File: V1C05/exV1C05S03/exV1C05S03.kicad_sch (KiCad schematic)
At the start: 4 parts

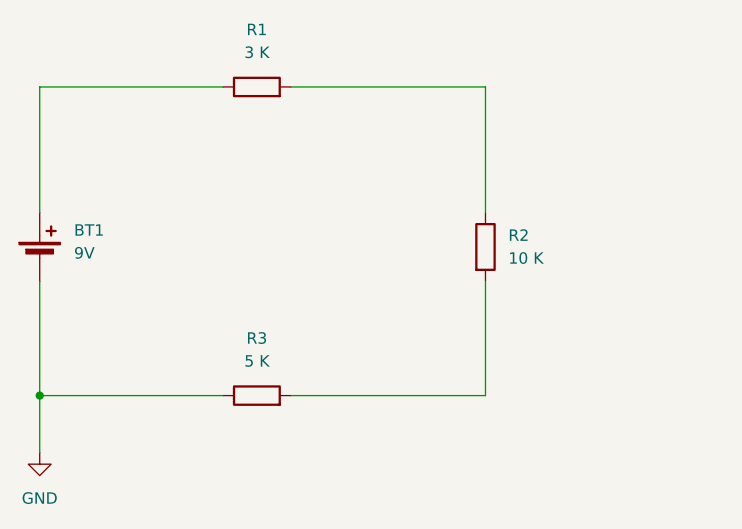
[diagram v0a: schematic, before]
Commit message: update exV1C05S03
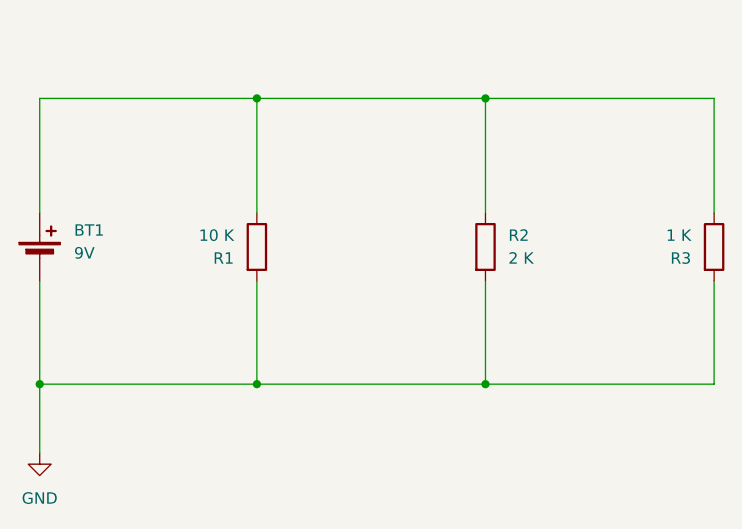
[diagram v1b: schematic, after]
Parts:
- R1: value 3 K -> 10 K
- R2: value 10 K -> 2 K
- R3: value 5 K -> 1 K
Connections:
- net GND: now also R1.2, R2.2, R3.2; no longer R3.1
- net at R2.1: now also BT1.1 (+), R1.1, R3.1; no longer R1.2
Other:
- moved on the sheet: R1, R3
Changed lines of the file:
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@@
 	(paper "A4")
 	(junction
-		(at 44.45 60.96)
-		(diameter 0)
-		(color 0 0 0 0)
-	)
-	(wire
-		(pts
-			(xy 72.39 26.67) (xy 93.98 26.67)
-		)
-		(stroke
-			(width 0)
-			(type default)
-		)
-	)
-	(wire
-		(pts
-			(xy 72.39 60.96) (xy 93.98 60.96)
-		)
-		(stroke
-			(width 0)
-			(type default)
-		)
-	)
-	(wire
-		(pts
-			(xy 44.45 60.96) (xy 64.77 60.96)
-		)
-		(stroke
-			(width 0)
-			(type default)
-		)
-	)
-	(wire
-		(pts
-			(xy 93.98 48.26) (xy 93.98 60.96)
-		)
-		(stroke
-			(width 0)
-			(type default)
-		)
-	)
-	(wire
-		(pts
-			(xy 44.45 48.26) (xy 44.45 60.96)
-		)
-		(stroke
-			(width 0)
-			(type default)
-		)
-	)
-	(wire
-		(pts
-			(xy 93.98 26.67) (xy 93.98 40.64)
-		)
-		(stroke
-			(width 0)
-			(type default)
-		)
-	)
-	(wire
-		(pts
-			(xy 44.45 60.96) (xy 44.45 67.31)
-		)
-		(stroke
-			(width 0)
-			(type default)
-		)
-	)
-	(wire
-		(pts
-			(xy 44.45 26.67) (xy 64.77 26.67)
-		)
-		(stroke
-			(width 0)
-			(type default)
-		)
-	)
-	(wire
-		(pts
-			(xy 44.45 40.64) (xy 44.45 26.67)
+		(at 68.58 27.94)
+		(diameter 0)
+		(color 0 0 0 0)
+	)
+	(junction
+		(at 68.58 59.69)
+		(diameter 0)
+		(color 0 0 0 0)
+	)
+	(junction
+		(at 44.45 59.69)
+		(diameter 0)
+		(color 0 0 0 0)
+	)
+	(junction
+		(at 93.98 59.69)
+		(diameter 0)
+		(color 0 0 0 0)
+	)
+	(junction
+		(at 93.98 27.94)
+		(diameter 0)
+		(color 0 0 0 0)
+	)
+	(wire
+		(pts
+			(xy 119.38 59.69) (xy 93.98 59.69)
+		)
+		(stroke
+			(width 0)
+			(type default)
+		)
+	)
+	(wire
+		(pts
+			(xy 44.45 27.94) (xy 68.58 27.94)
+		)
+		(stroke
+			(width 0)
+			(type default)
+		)
+	)
+	(wire
+		(pts
+			(xy 119.38 27.94) (xy 119.38 40.64)
+		)
+		(stroke
+			(width 0)
+			(type default)
+		)
+	)
+	(wire
+		(pts
+			(xy 68.58 48.26) (xy 68.58 59.69)
+		)
+		(stroke
+			(width 0)
+			(type default)
+		)
+	)
+	(wire
+		(pts
+			(xy 119.38 48.26) (xy 119.38 59.69)
+		)
+		(stroke
+			(width 0)
+			(type default)
+		)
+	)
+	(wire
+		(pts
+			(xy 93.98 27.94) (xy 93.98 40.64)
+		)
+		(stroke
+			(width 0)
+			(type default)
+		)
+	)
+	(wire
+		(pts
+			(xy 44.45 48.26) (xy 44.45 59.69)
+		)
+		(stroke
+			(width 0)
+			(type default)
+		)
+	)
+	(wire
+		(pts
+			(xy 68.58 59.69) (xy 93.98 59.69)
+		)
+		(stroke
+			(width 0)
+			(type default)
+		)
+	)
+	(wire
+		(pts
+			(xy 44.45 59.69) (xy 44.45 67.31)
+		)
+		(stroke
+			(width 0)
+			(type default)
+		)
+	)
+	(wire
+		(pts
+			(xy 93.98 27.94) (xy 119.38 27.94)
+		)
+		(stroke
+			(width 0)
+			(type default)
+		)
+	)
+	(wire
+		(pts
+			(xy 44.45 59.69) (xy 68.58 59.69)
+		)
+		(stroke
+			(width 0)
+			(type default)
+		)
+	)
+	(wire
+		(pts
+			(xy 93.98 59.69) (xy 93.98 48.26)
+		)
+		(stroke
+			(width 0)
+			(type default)
+		)
+	)
+	(wire
+		(pts
+			(xy 44.45 27.94) (xy 44.45 40.64)
+		)
+		(stroke
+			(width 0)
+			(type default)
+		)
+	)
+	(wire
+		(pts
+			(xy 68.58 27.94) (xy 93.98 27.94)
+		)
+		(stroke
+			(width 0)
+			(type default)
+		)
+	)
+	(wire
+		(pts
+			(xy 68.58 27.94) (xy 68.58 40.64)
 		)
 		(stroke
@@
 			)
 		)
-		(property "Value" "10 K"
+		(property "Value" "2 K"
 			(at 96.52 45.7199 0)
 			(effects
@@
 	(symbol
 		(lib_id "Device:R")
-		(at 68.58 26.67 90)
+		(at 68.58 44.45 0)
 		(unit 1)
 		(exclude_from_sim no)
@@
 		(fields_autoplaced yes)
 		(property "Reference" "R1"
-			(at 68.58 20.32 90)
-			(effects
-				(font
-					(size 1.27 1.27)
-				)
-			)
-		)
-		(property "Value" "3 K"
-			(at 68.58 22.86 90)
-			(effects
-				(font
-					(size 1.27 1.27)
-				)
+			(at 66.04 45.7201 0)
+			(effects
+				(font
+					(size 1.27 1.27)
+				)
+				(justify right)
+			)
+		)
+		(property "Value" "10 K"
+			(at 66.04 43.1801 0)
+			(effects
+				(font
+					(size 1.27 1.27)
+				)
+				(justify right)
 			)
 		)
 		(property "Footprint" ""
-			(at 68.58 28.448 90)
+			(at 66.802 44.45 90)
 			(effects
 				(font
@@
 		)
 		(property "Datasheet" "~"
-			(at 68.58 26.67 0)
+			(at 68.58 44.45 0)
 			(effects
 				(font
@@
 		)
 		(property "Description" "Resistor"
-			(at 68.58 26.67 0)
+			(at 68.58 44.45 0)
 			(effects
 				(font
@@
 	(symbol
 		(lib_id "Device:R")
-		(at 68.58 60.96 90)
+		(at 119.38 44.45 0)
 		(unit 1)
 		(exclude_from_sim no)
@@
 		(fields_autoplaced yes)
 		(property "Reference" "R3"
-			(at 68.58 54.61 90)
-			(effects
-				(font
-					(size 1.27 1.27)
-				)
-			)
-		)
-		(property "Value" "5 K"
-			(at 68.58 57.15 90)
-			(effects
-				(font
-					(size 1.27 1.27)
-				)
+			(at 116.84 45.7201 0)
+			(effects
+				(font
+					(size 1.27 1.27)
+				)
+				(justify right)
+			)
+		)
+		(property "Value" "1 K"
+			(at 116.84 43.1801 0)
+			(effects
+				(font
+					(size 1.27 1.27)
+				)
+				(justify right)
 			)
 		)
 		(property "Footprint" ""
-			(at 68.58 62.738 90)
+			(at 117.602 44.45 90)
 			(effects
 				(font
@@
 		)
 		(property "Datasheet" "~"
-			(at 68.58 60.96 0)
+			(at 119.38 44.45 0)
 			(effects
 				(font
@@
 		)
 		(property "Description" "Resistor"
-			(at 68.58 60.96 0)
-			(effects
-				(font
+			(at 119.38 44.45 0)
+			(effects
+				(font
